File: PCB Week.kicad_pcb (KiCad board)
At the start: 2 copper layers, 80.2 x 98.4 mm, 7 parts, among them J1 Conn_01x04_Pin, J2 Conn_01x08_Pin, SW1 SW_Push, SW2 SW_Push, U1 XIAO-ESP32-C3-SMD, U2 DHT11

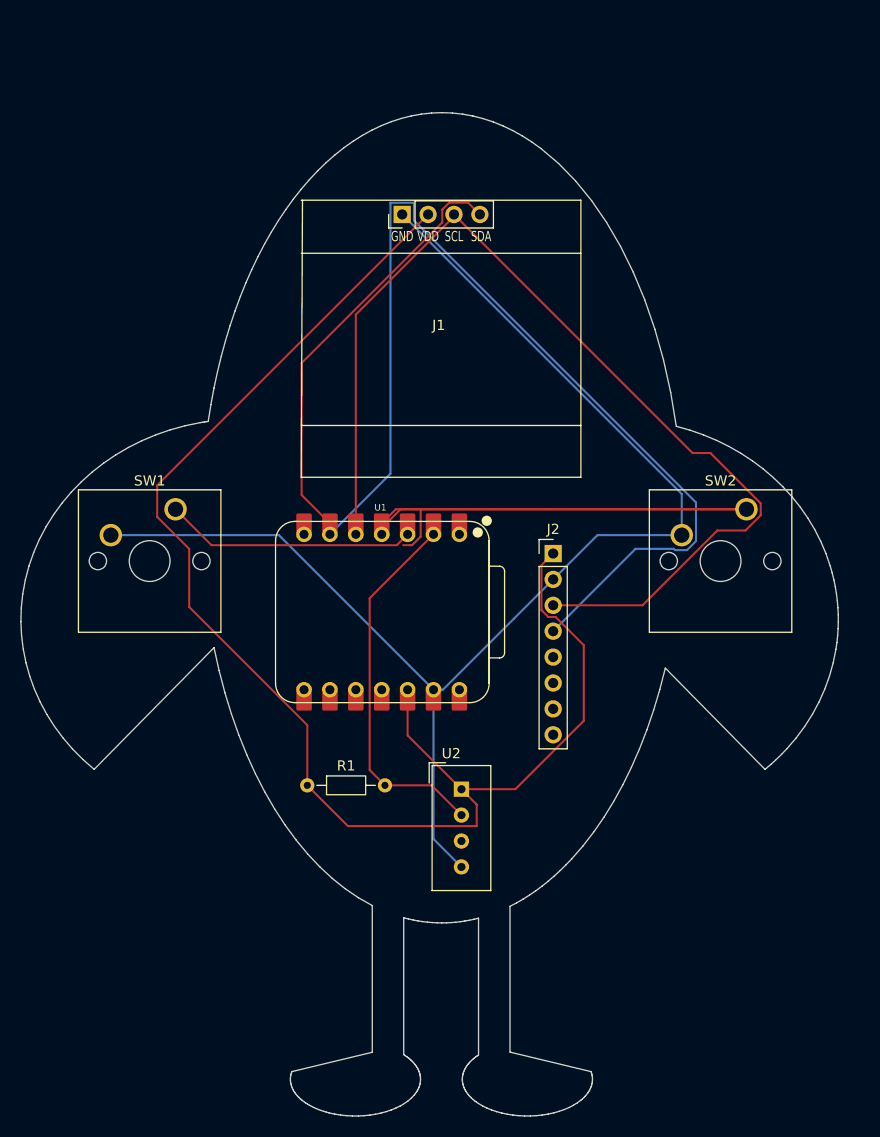
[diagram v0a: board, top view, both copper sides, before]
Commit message: Updates on wiring and layout
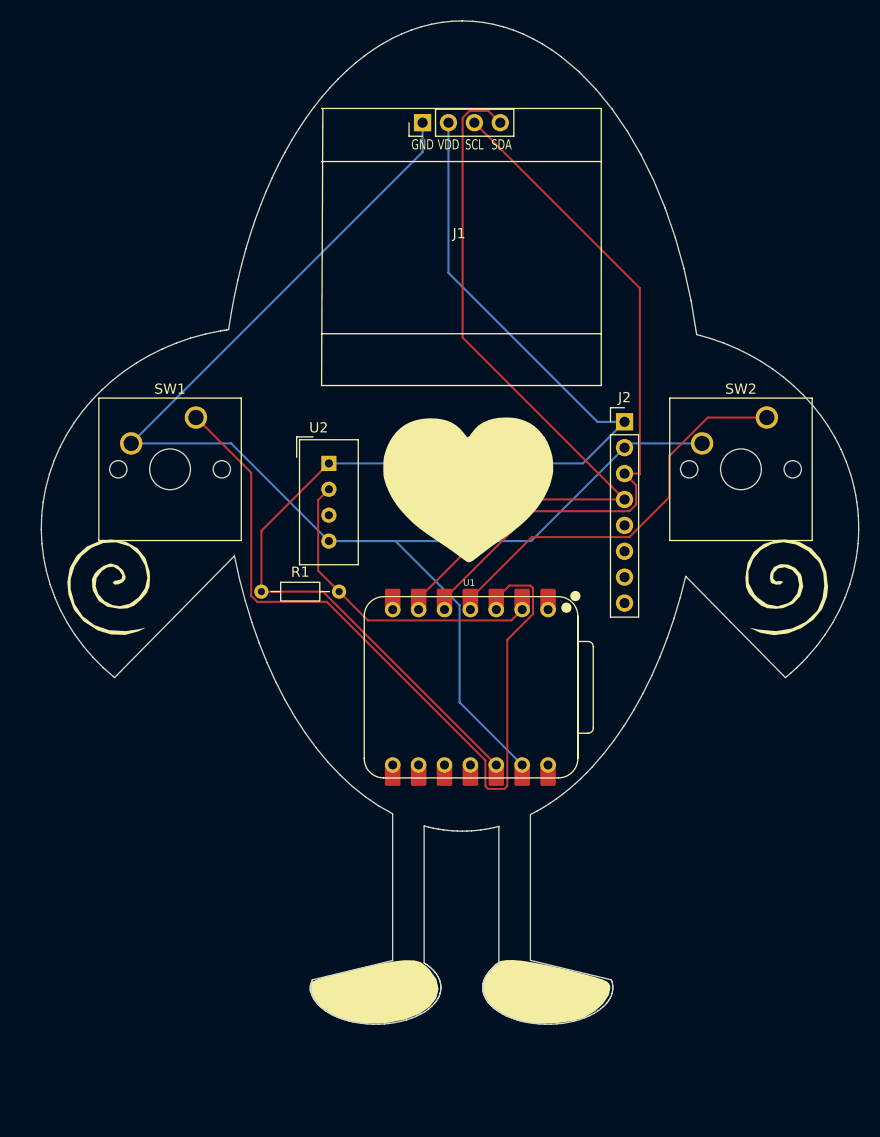
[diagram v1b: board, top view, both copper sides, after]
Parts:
- added G***: LOGO, LOGO, F.Cu at (142.5, 98.5)
- added G***: LOGO, LOGO, F.Cu at (145.0, 95.5)
- added G***: LOGO, LOGO, F.Cu at (142.5, 97.5)
- moved U2 34.5 mm to (131.5, 92.9)
- moved R1 19.5 mm to (124.9, 105.5)
- moved J2 14.7 mm to (160.5, 88.8)
- moved U1 11.4 mm to (145.4, 114.9)
- moved J1 9.22 mm to (144.5, 59.5)
- moved SW1 9.22 mm to (118.5, 88.4)
- moved SW2 9.22 mm to (174.5, 88.4)
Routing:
- net /SDA: track 141.8 -> 73.8 mm
- net /GPIO2: track 24.7 -> 81.1 mm
- net /GPIO3: track 78.3 -> 39.9 mm
- net /SCL: track 102.2 -> 70.0 mm
- net +3.3V: track 141.4 -> 114.1 mm
- net GND: track 129.9 -> 139.9 mm
- net /DHT11 DATA: track 36.5 -> 30.9 mm

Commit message: 3D images
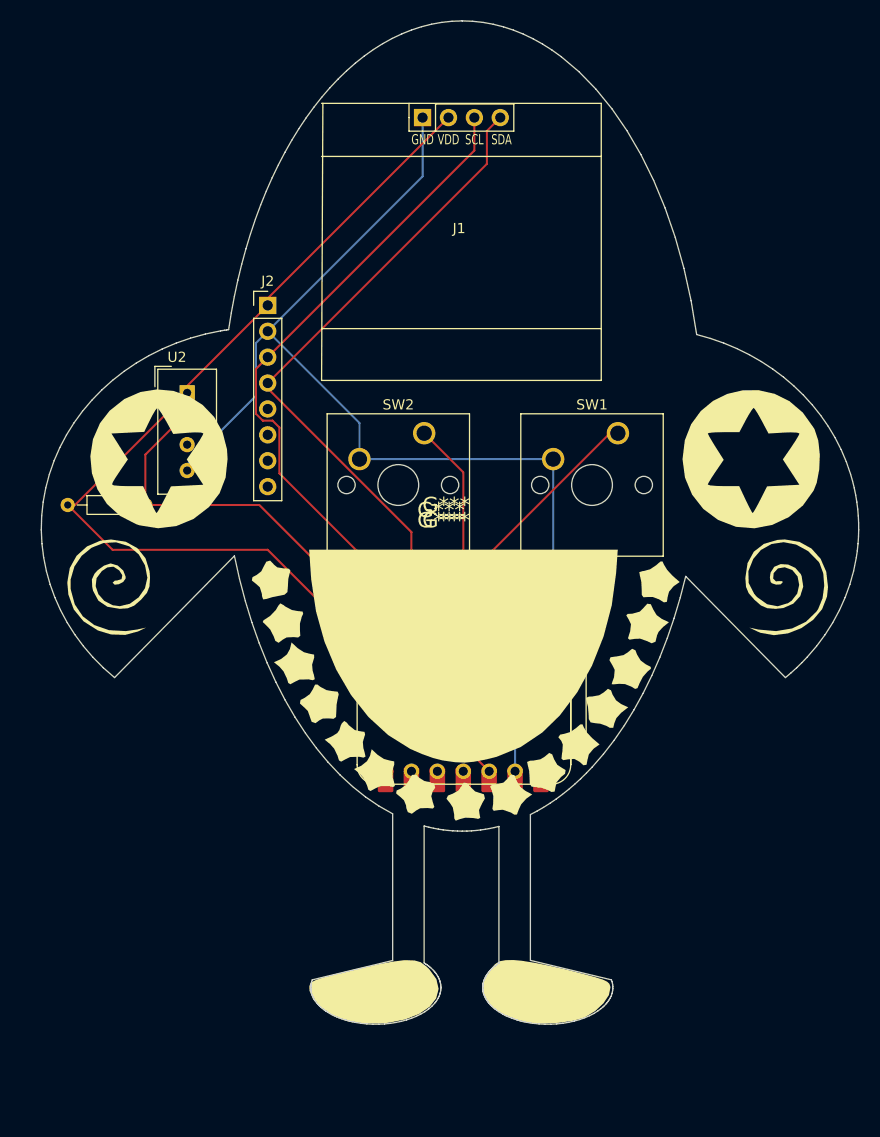
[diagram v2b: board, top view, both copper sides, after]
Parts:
- removed the G*** at (145.0, 95.5)
- added G***: LOGO, LOGO, F.Cu at (143.0, 97.0)
- added G***: LOGO, LOGO, F.Cu at (143.0, 98.5)
- added G***: LOGO, Starbie:backside, B.Cu at (145.0, 96.5)
- moved SW1 41.4 mm to (159.8, 90.0)
- moved J2 36.8 mm to (125.5, 77.4)
- moved SW2 33.6 mm to (140.8, 90.0)
- moved R1 20.8 mm to (105.9, 97.0)
- moved U2 15.5 mm to (117.6, 86.0)
- moved U1 0.93 mm to (144.7, 115.5)
- moved J1 0.50 mm to (144.5, 59.0)
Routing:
- net /GPIO2: track 81.1 -> 23.6 mm
- net GND: track 139.9 -> 111.0 mm
- net /DHT11 DATA: track 30.9 -> 52.7 mm
- net /GPIO3: track 39.9 -> 19.5 mm
- net /SDA: track 73.8 -> 64.2 mm
- net +3.3V: track 114.1 -> 106.1 mm
- net /SCL: track 70.0 -> 68.9 mm
